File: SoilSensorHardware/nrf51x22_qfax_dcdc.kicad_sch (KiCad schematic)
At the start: 36 parts, among them J1 Conn_02x07_Odd_Even, J2 Conn_01x06, U1 nrf52810-QFAA-T, U2 TLC555xD, X1 Crystal-4, X2 32.768kHz

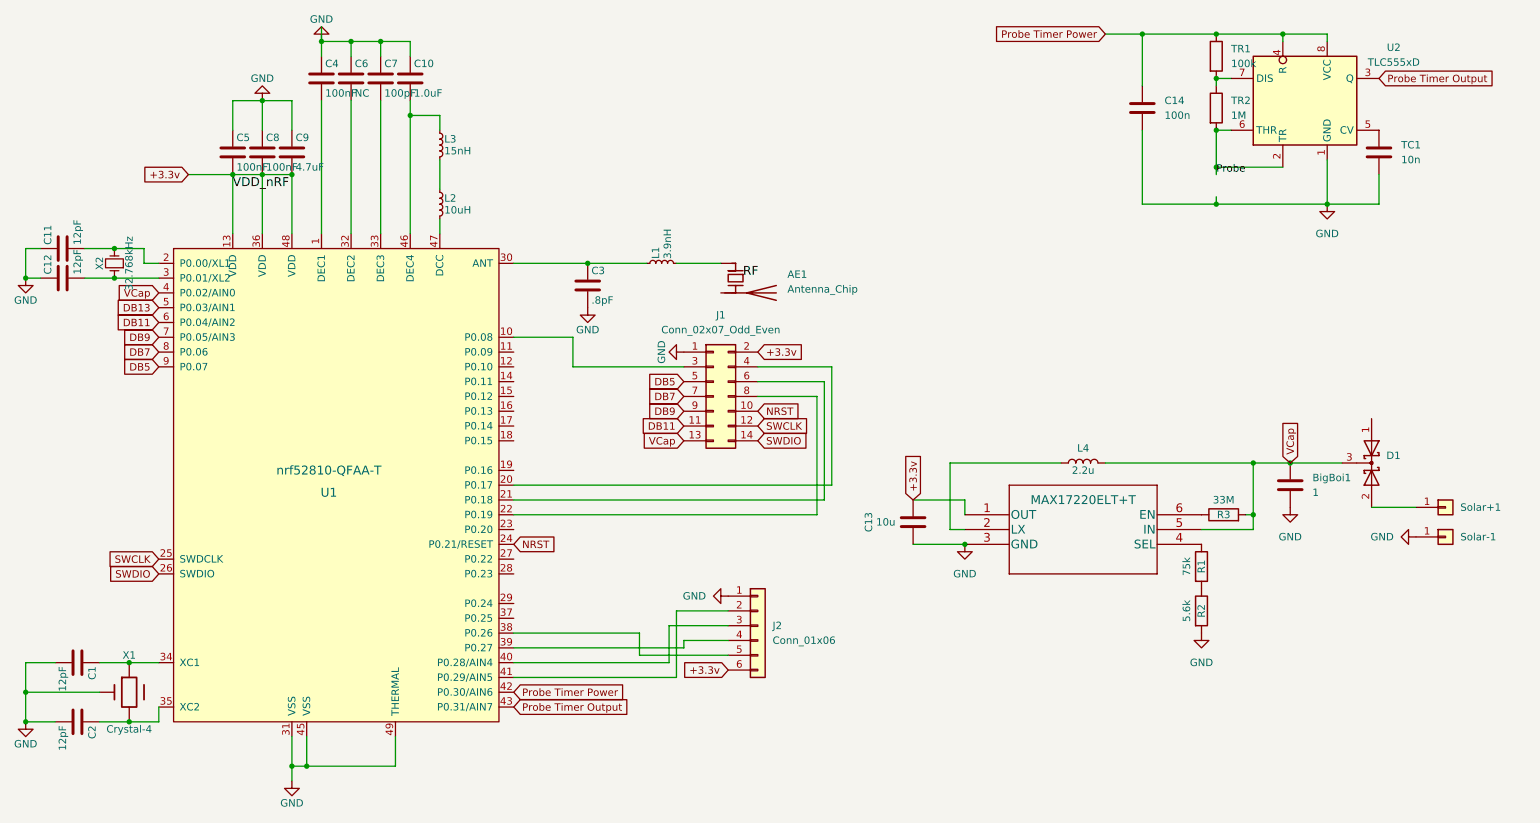
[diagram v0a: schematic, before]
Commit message: Updated schematic
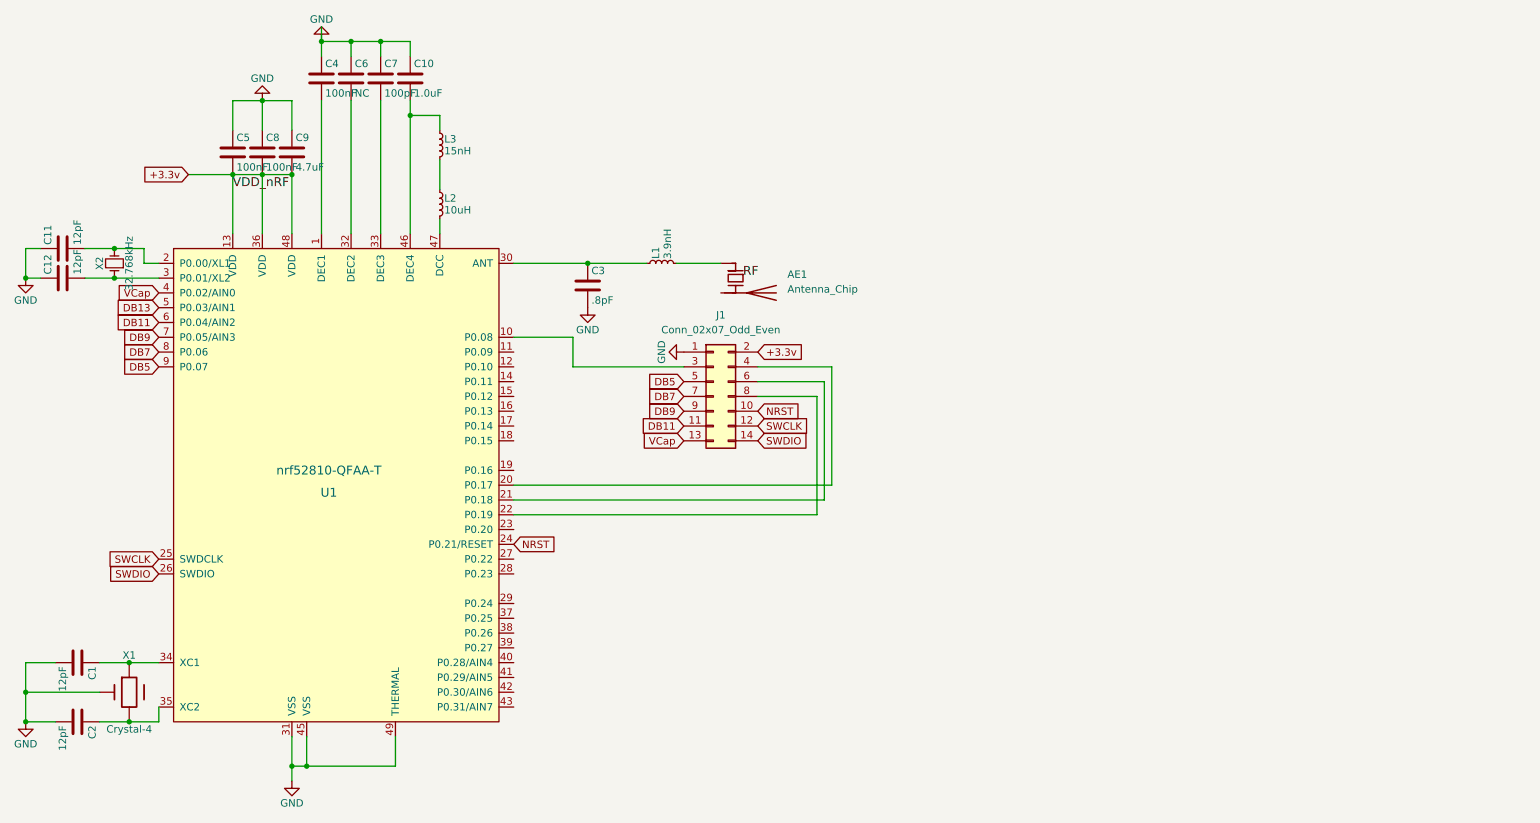
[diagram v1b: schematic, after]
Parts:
- removed BigBoi1: 1, Capacitor_THT:CP_Radial_D6.3mm_P2.50mm, symbol Device:C
- removed C13: 10u, Inductor_SMD:L_0603_1608Metric, symbol Device:C
- removed C14: 100n, Capacitor_SMD:C_0402_1005Metric, symbol Device:C
- removed D1: BAT54C,215, Package_TO_SOT_SMD:SOT-23, symbol Device:D_Schottky_Dual_CommonCathode_AAK
- removed DCDC1: MAX17220ELT+T, Custom:MAX17220ELT&plus_T, symbol Custom_Symbols:MAX17220ELT+T
- removed J2: Conn_01x06, Connector_PinHeader_2.54mm:PinHeader_1x06_P2.54mm_Vertical, symbol Connector_Generic:Conn_01x06
- removed L4: 2.2u, Inductor_SMD:L_0805_2012Metric, symbol Device:L
- removed R1: 75k, Resistor_SMD:R_0603_1608Metric, symbol Device:R
- removed R2: 5.6k, Resistor_SMD:R_0603_1608Metric, symbol Device:R
- removed R3: 33M, Resistor_SMD:R_0603_1608Metric, symbol Device:R
- removed Solar+1, Solar-1: Conn_01x01, Connector_PinHeader_2.54mm:PinHeader_1x01_P2.54mm_Vertical, symbol Connector_Generic:Conn_01x01
- removed TC1: 10n, Capacitor_SMD:C_0603_1608Metric, symbol Device:C
- removed TR1: 100k, Resistor_SMD:R_0805_2012Metric, symbol Device:R
- removed TR2: 1M, Resistor_SMD:R_0805_2012Metric, symbol Device:R
- removed U2: TLC555xD, Package_SO:SOIC-8_3.9x4.9mm_P1.27mm, symbol Timer:TLC555xD
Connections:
- net Probe Timer Output: no longer names the net of U1.43 (P0.31/AIN7)
- net Probe Timer Power: no longer names the net of U1.42 (P0.30/AIN6)
